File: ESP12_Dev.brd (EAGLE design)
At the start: 37.5 x 37.1 mm, 11 parts

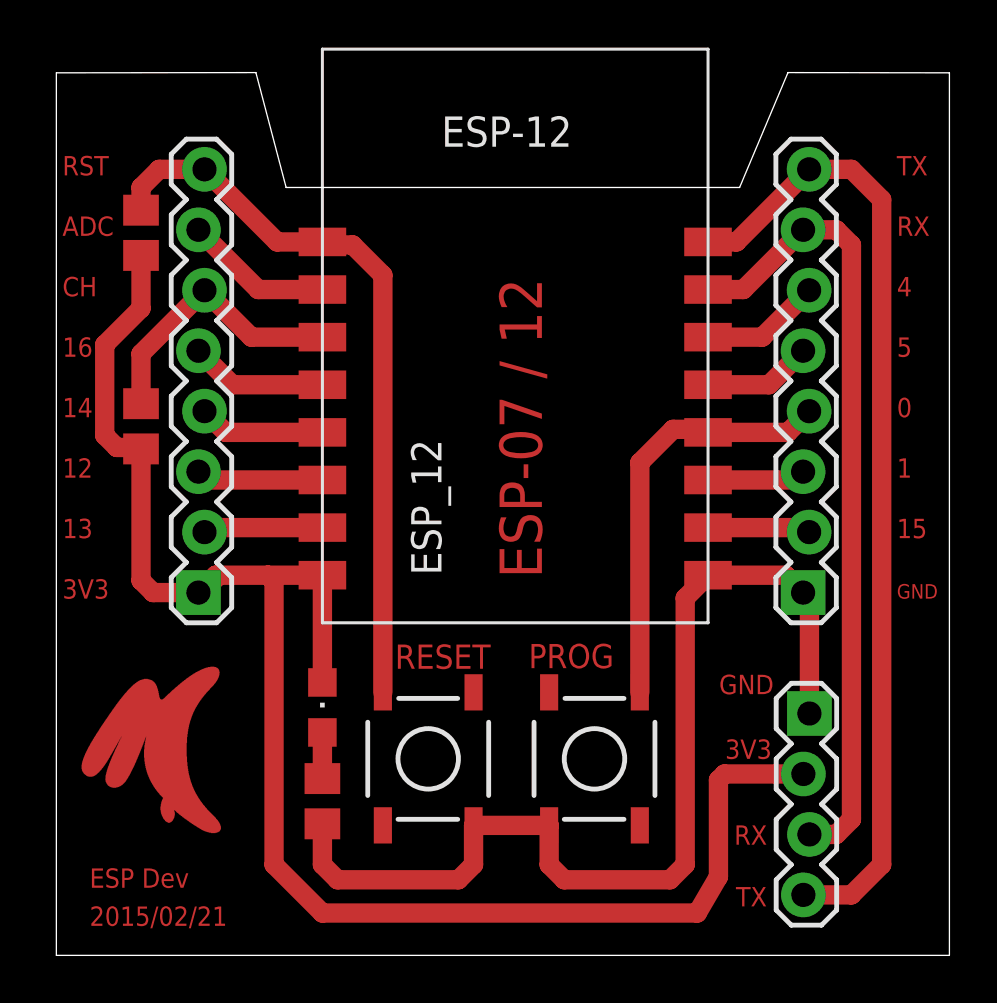
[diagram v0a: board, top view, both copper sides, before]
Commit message: Version one
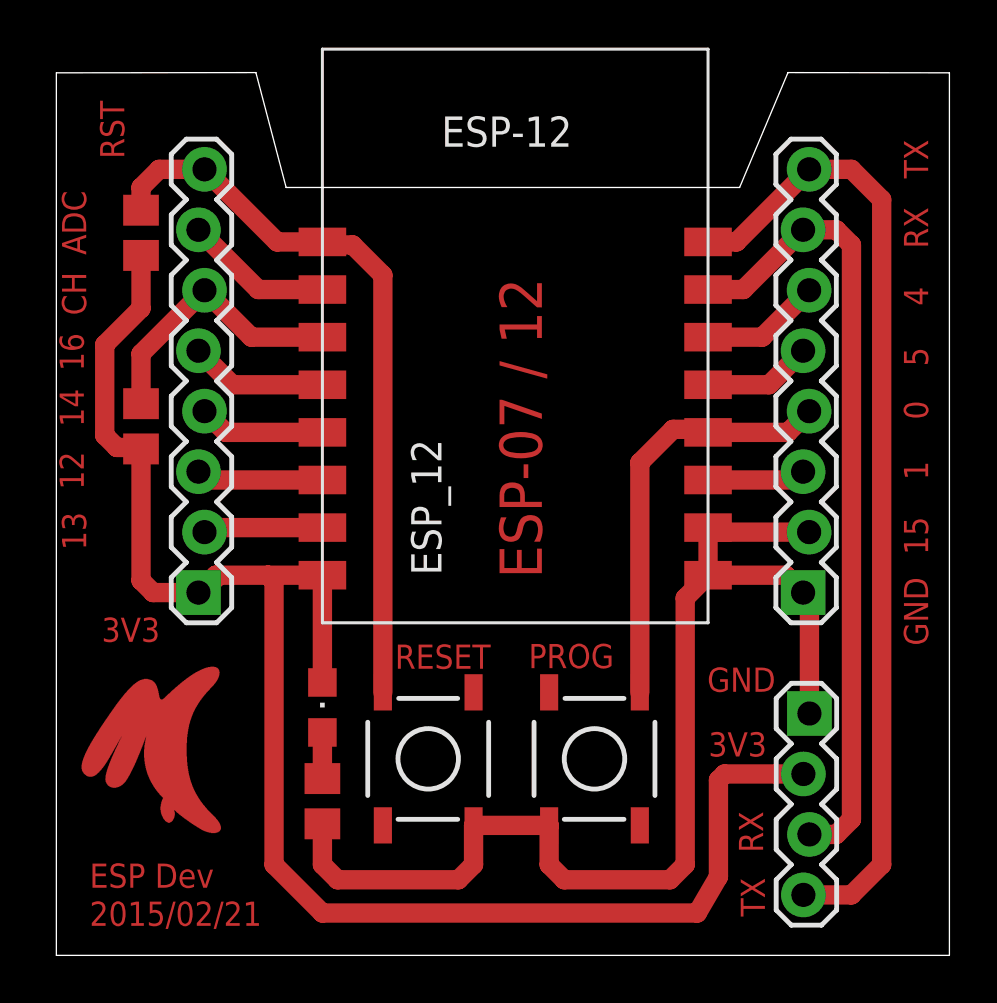
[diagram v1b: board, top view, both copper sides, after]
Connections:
- removed net GPIO15: ESP_12.2, JP2.2
- net GND: now also ESP_12.2, JP2.2
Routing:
- net GND: track 43.4 -> 49.8 mm
- net GPIO15: track 4.33 -> 0.00 mm
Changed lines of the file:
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@@
 <text x="26.4414" y="22.225" size="1.016" layer="1">PROG</text>
 <text x="20.828" y="22.1996" size="1.016" layer="1">RESET</text>
-<text x="35.0774" y="14.8082" size="0.8128" layer="1">RX</text>
-<text x="35.1536" y="12.2174" size="0.8128" layer="1">TX</text>
-<text x="34.4424" y="21.1328" size="0.8128" layer="1">GND</text>
-<text x="34.6964" y="18.415" size="0.8128" layer="1">3V3</text>
-<text x="6.858" y="42.926" size="0.8128" layer="1">RST</text>
-<text x="6.858" y="40.386" size="0.8128" layer="1">ADC</text>
-<text x="6.858" y="37.846" size="0.8128" layer="1">CH</text>
-<text x="6.858" y="35.306" size="0.8128" layer="1">16</text>
-<text x="6.858" y="32.766" size="0.8128" layer="1">14</text>
-<text x="6.858" y="30.226" size="0.8128" layer="1">12</text>
-<text x="6.858" y="27.686" size="0.8128" layer="1">13</text>
-<text x="6.858" y="25.146" size="0.8128" layer="1">3V3</text>
-<text x="41.91" y="37.846" size="0.8128" layer="1">4</text>
-<text x="41.91" y="42.926" size="0.8128" layer="1">TX</text>
-<text x="41.91" y="40.386" size="0.8128" layer="1">RX</text>
-<text x="41.91" y="35.306" size="0.8128" layer="1">5</text>
-<text x="41.91" y="32.766" size="0.8128" layer="1">0</text>
-<text x="41.91" y="30.226" size="0.8128" layer="1">1</text>
-<text x="41.91" y="27.686" size="0.8128" layer="1">15</text>
-<text x="41.91" y="25.146" size="0.6096" layer="1">GND</text>
+<text x="35.2774" y="16.2082" size="1.016" layer="1" rot="R270">RX</text>
+<text x="35.3536" y="13.4174" size="1.016" layer="1" rot="R270">TX</text>
+<text x="33.9424" y="21.2328" size="1.016" layer="1">GND</text>
+<text x="33.9964" y="18.515" size="1.016" layer="1">3V3</text>
+<text x="9.458" y="43.626" size="1.016" layer="1" rot="R90">RST</text>
+<text x="7.858" y="39.586" size="1.016" layer="1" rot="R90">ADC</text>
+<text x="7.858" y="37.046" size="1.016" layer="1" rot="R90">CH</text>
+<text x="7.758" y="34.706" size="1.016" layer="1" rot="R90">16</text>
+<text x="7.758" y="32.366" size="1.016" layer="1" rot="R90">14</text>
+<text x="7.758" y="29.726" size="1.016" layer="1" rot="R90">12</text>
+<text x="7.858" y="27.186" size="1.016" layer="1" rot="R90">13</text>
+<text x="10.958" y="24.346" size="1.016" layer="1" distance="54" rot="R180">3V3</text>
+<text x="42.21" y="38.246" size="1.016" layer="1" rot="R270">4</text>
+<text x="42.21" y="44.426" size="1.016" layer="1" rot="R270">TX</text>
+<text x="42.21" y="41.586" size="1.016" layer="1" rot="R270">RX</text>
+<text x="42.21" y="35.706" size="1.016" layer="1" rot="R270">5</text>
+<text x="42.21" y="33.466" size="1.016" layer="1" rot="R270">0</text>
+<text x="42.21" y="30.926" size="1.016" layer="1" rot="R270">1</text>
+<text x="42.21" y="28.586" size="1.016" layer="1" rot="R270">15</text>
+<text x="42.21" y="26.046" size="1.016" layer="1" rot="R270">GND</text>
 <text x="27" y="26" size="1.778" layer="1" rot="R90">ESP-07 / 12</text>
-<text x="8" y="11.4" size="0.8128" layer="1">2015/02/21</text>
-<text x="8" y="13" size="0.8128" layer="1">ESP Dev</text>
+<text x="8" y="11.4" size="1.016" layer="1">2015/02/21</text>
+<text x="8" y="13" size="1.016" layer="1">ESP Dev</text>
 </plain>
 <attributes>
@@
 <wire x1="33.02" y1="13.97" x2="33.02" y2="25.17" width="0.8128" layer="1"/>
 <wire x1="33.02" y1="25.17" x2="33.98" y2="26.13" width="0.8128" layer="1"/>
+<contactref element="ESP_12" pad="2"/>
+<contactref element="JP2" pad="2"/>
+<wire x1="33.98" y1="28.13" x2="33.98" y2="26.13" width="0.8128" layer="1"/>
+<wire x1="38.227" y1="27.94" x2="33.98" y2="27.94" width="0.8128" layer="1"/>
+<wire x1="33.98" y1="27.94" x2="33.98" y2="28.13" width="0.8128" layer="1"/>
 </signal>
 <signal name="GPIO13">
@@
 <wire x1="10.16" y1="35.433" x2="12.827" y2="38.1" width="0.8128" layer="1"/>
 </signal>
-<signal name="GPIO15">
-<contactref element="ESP_12" pad="2"/>
-<contactref element="JP2" pad="2"/>
-<wire x1="33.98" y1="28.13" x2="38.037" y2="28.13" width="0.8128" layer="1"/>
-<wire x1="38.037" y1="28.13" x2="38.227" y2="27.94" width="0.8128" layer="1"/>
-</signal>
 <signal name="N$1">
